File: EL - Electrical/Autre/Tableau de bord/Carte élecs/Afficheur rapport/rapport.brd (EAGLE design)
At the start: 54.9 x 40.9 mm, 15 parts, among them IC1 MCP23008P, X1 22-23-2041

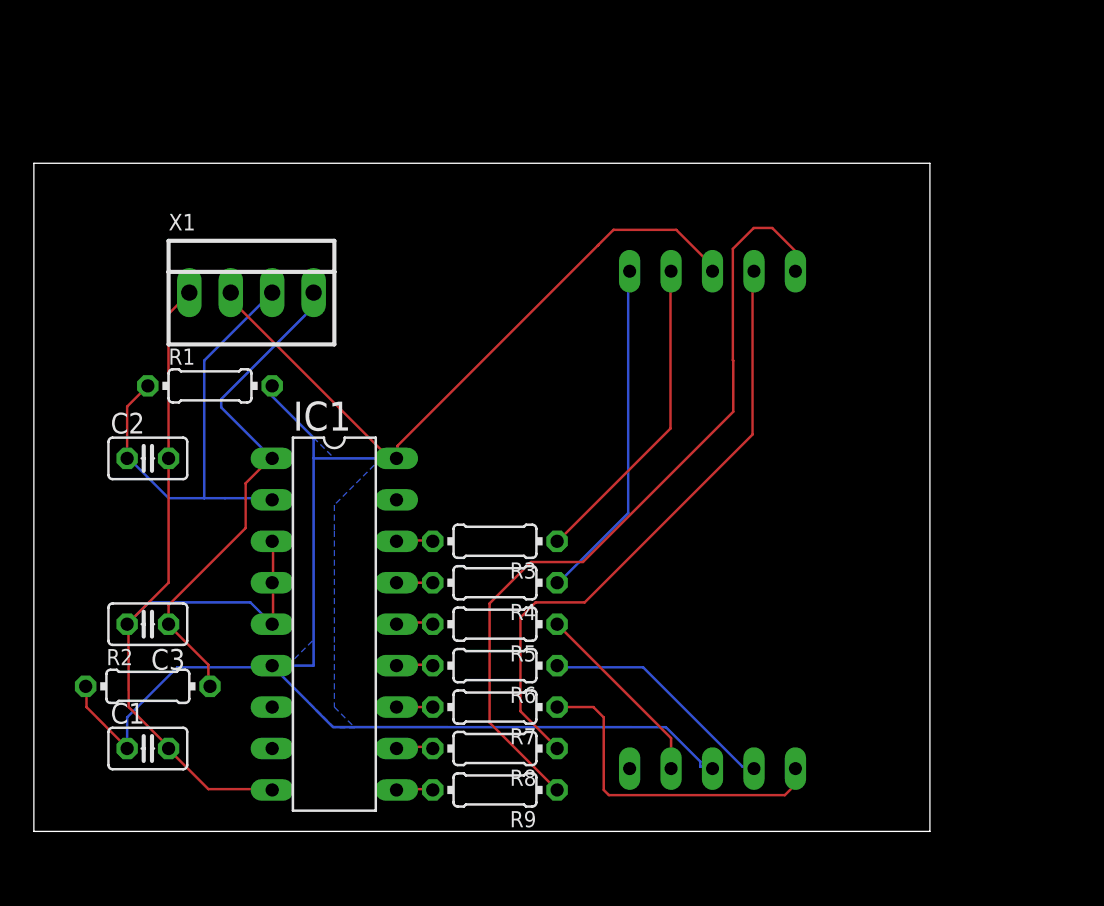
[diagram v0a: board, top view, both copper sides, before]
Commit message: Afficheur rapport maj
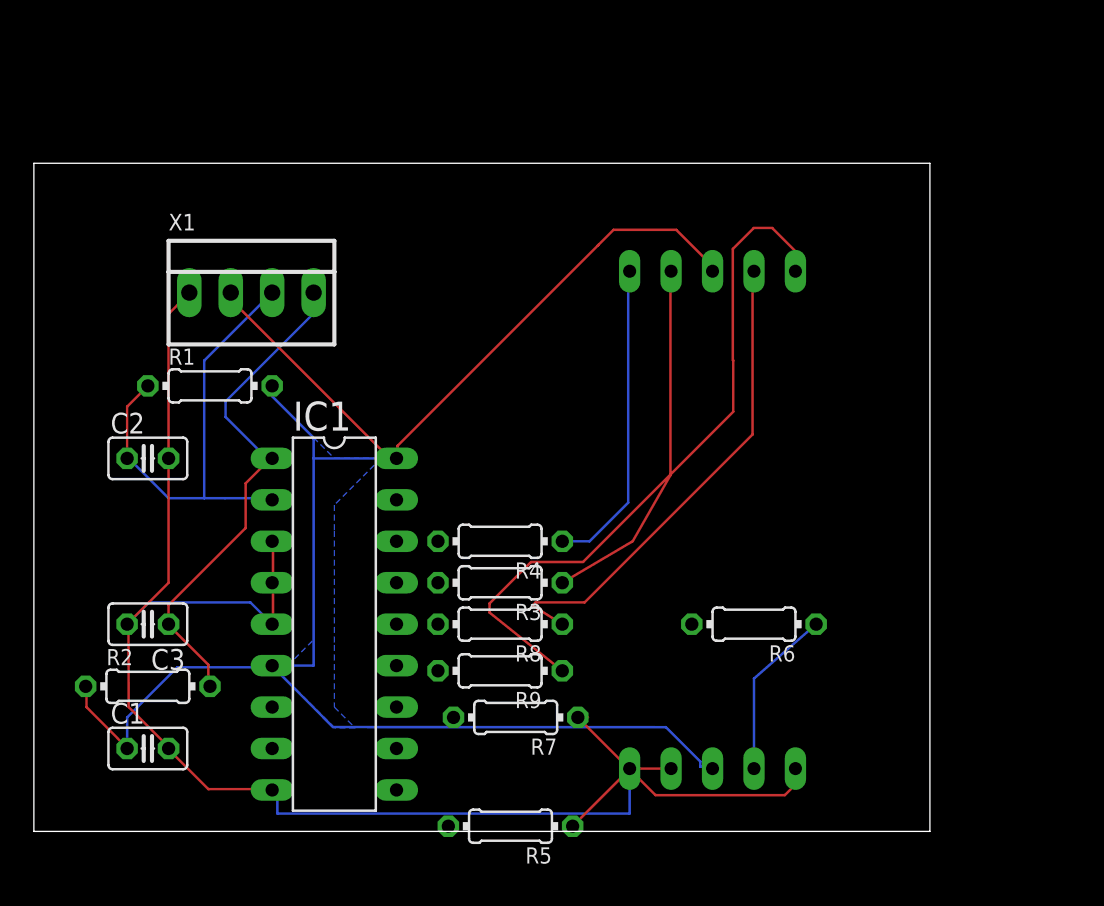
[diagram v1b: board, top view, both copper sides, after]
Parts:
- moved R6 16.1 mm to (44.1, 12.7)
- moved R5 12.4 mm to (29.2, 0.32)
- moved R8 7.63 mm to (28.6, 12.7)
- moved R9 7.31 mm to (28.6, 9.84)
- moved R3 2.56 mm to (28.6, 15.2)
- moved R4 2.56 mm to (28.6, 17.8)
- moved R7 1.42 mm to (29.5, 6.99)
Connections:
- net N$8 renamed SCL
- net N$9 renamed SDA
- removed net N$1: IC1.16, R3.2
- removed net N$3: IC1.14, R5.2
- removed net N$4: IC1.13, R6.2
- removed net N$6: IC1.11, R8.2
- removed net N$7: IC1.10, R9.2
- new net GP0: IC1.10, R5.2
- new net GP1: IC1.11
- new net GP2: IC1.12
- new net GP3: IC1.13, R7.2
- new net GP4: IC1.14, R8.2
- new net GP5: IC1.15, R3.2
- new net GP6: IC1.16, R4.2
- net GND: now also LED1.5
- net N$2: now also R9.2; no longer IC1.15, R4.2
- net N$5: now also R6.2; no longer IC1.12, R7.2
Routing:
- net GND: track 53.6 -> 79.6 mm
- net N$11: track 37.9 -> 30.1 mm
- net N$10: track 49.1 -> 42.2 mm
- net N$14: track 11.9 -> 7.60 mm
- net N$12: track 21.3 -> 17.2 mm
- net N$13: track 14.7 -> 10.6 mm
- net N$16: track 19.5 -> 22.2 mm
- net N$3: track 2.36 -> 0.00 mm
- net N$6: track 2.36 -> 0.00 mm
- net N$4: track 2.27 -> 0.00 mm
- net N$7: track 2.27 -> 0.00 mm
- net N$1: track 2.27 -> 0.00 mm
- net N$5: track 2.22 -> 0.00 mm
- net N$2: track 2.22 -> 0.00 mm
- net N$15: track 21.0 -> 19.3 mm

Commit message: carte afficheur rapport et commandes
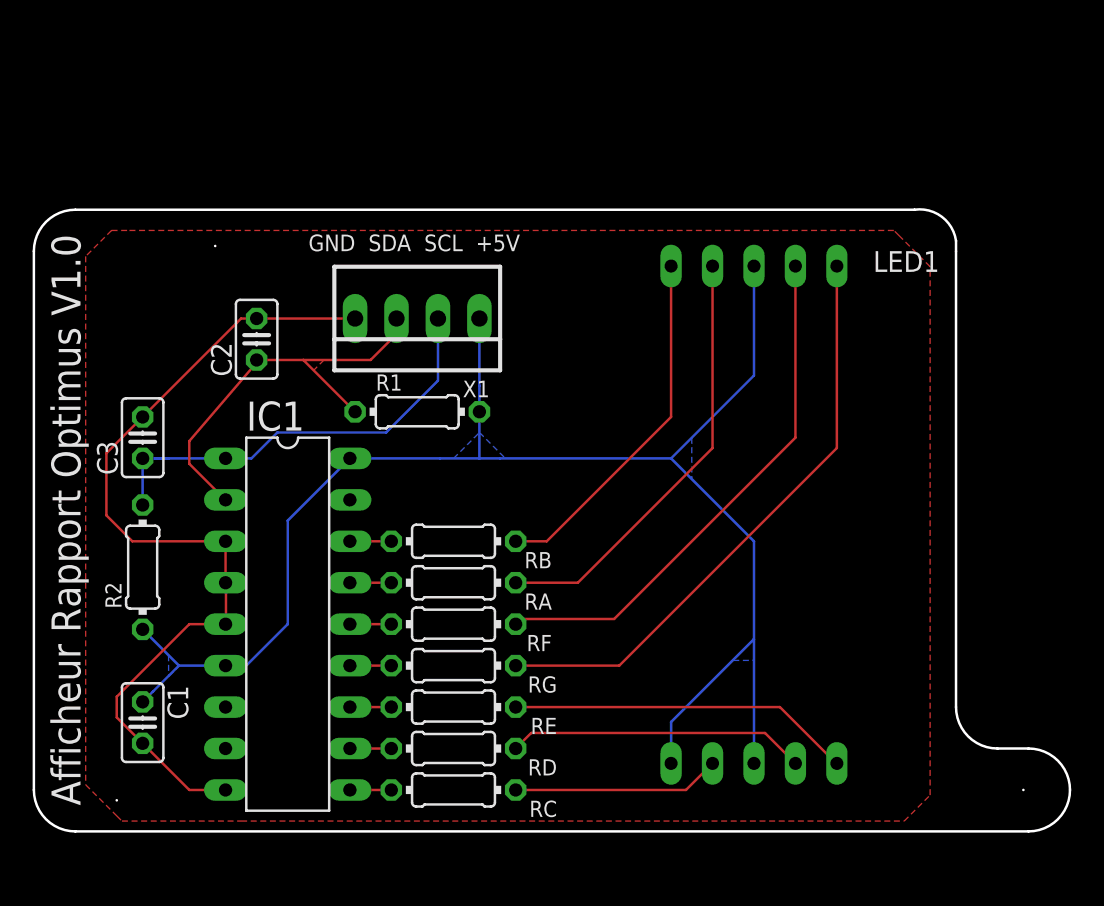
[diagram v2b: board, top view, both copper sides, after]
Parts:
- removed R3, R4, R5, R6, R7, R8, R9: 470, rcl:0204/7
- added RA, RB, RC, RD, RE, RF, RG: 470, rcl:0204/7
- moved R1 12.8 mm to (23.5, 25.7)
- moved C3 11.4 mm to (6.67, 24.1), turned to 90 degrees
- moved X1 10.3 mm to (23.5, 31.4), turned to 180 degrees
- moved C2 9.89 mm to (13.7, 30.2), turned to 90 degrees
- moved R2 7.31 mm to (6.67, 16.2), turned to 90 degrees
- moved IC1 2.86 mm to (15.6, 12.7)
- moved LED1 2.56 mm to (44.1, 19.4)
- moved C1 1.62 mm to (6.67, 6.67), turned to 270 degrees
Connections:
- removed net N$2: R9.2
- removed net N$5: R6.2
- net +5V: now also LED1.5, X1.1; no longer X1.2
- net GND: now also X1.4; no longer LED1.5, X1.1
- net GP0: now also RC.2; no longer R5.2
- net GP1: now also RD.2
- net GP2: now also RE.2
- net GP3: now also RG.2; no longer R7.2
- net GP4: now also RF.2; no longer R8.2
- net GP5: now also RA.2; no longer R3.2
- net GP6: now also RB.2; no longer R4.2
- net N$10: now also RG.1; no longer R9.1
- net N$11: now also RF.1; no longer R8.1
- net N$12: now also RE.1; no longer R7.1
- net N$13: now also RD.1; no longer R6.1
- net N$14: now also RC.1; no longer R5.1
- net N$15: now also RB.1; no longer R4.1
- net N$16: now also RA.1; no longer R3.1
- net SCL: now also X1.2; no longer X1.4
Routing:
- net GND: track 79.6 -> 53.8 mm
- net +5V: track 114.5 -> 99.7 mm
- net N$13: track 10.6 -> 18.3 mm
- net N$10: track 42.2 -> 36.4 mm
- net N$14: track 7.60 -> 12.8 mm
- net N$12: track 17.2 -> 21.7 mm
- net N$16: track 22.2 -> 26.6 mm
- net SCL: track 31.4 -> 27.7 mm
- net SDA: track 29.1 -> 25.7 mm
- net N$15: track 19.3 -> 21.9 mm
- net GP6: track 0.00 -> 2.54 mm
- net GP5: track 0.00 -> 2.54 mm
- net GP4: track 0.00 -> 2.54 mm
- net GP3: track 0.00 -> 2.54 mm
- net GP2: track 0.00 -> 2.54 mm
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- added copper zone on layer 1, net GND
- added copper zone on layer 1, net SDA
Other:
- board size 54.9 x 40.9 mm -> 63.5 x 38.1 mm
- board text added: "Afficheur Rapport Optimus V1.0"
- board text added: "GND SDA SCL +5V"
